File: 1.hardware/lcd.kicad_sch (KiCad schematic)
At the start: 36 parts, among them J6 FPC_LCD_40

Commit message: 중간 저장
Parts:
- PS1, PS2: footprint SOT65P210X110-5N -> SamacSys_Parts:SOT65P210X110-5N
- R12, R13, R14, R15, R16, R17, R18, R19, R20, R21, R22, R23, R24, R25, R26, R27, R28, R29, R30, R31, R32, R33: footprint (none) -> Resistor_SMD:R_0402_1005Metric
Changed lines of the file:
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@@
 			)
 		)
-		(property "Footprint" ""
+		(property "Footprint" "Resistor_SMD:R_0402_1005Metric"
 			(at 204.47 48.26 0)
 			(effects
@@
 			)
 		)
-		(property "Footprint" ""
+		(property "Footprint" "Resistor_SMD:R_0402_1005Metric"
 			(at 204.47 50.8 0)
 			(effects
@@
 			)
 		)
-		(property "Footprint" ""
+		(property "Footprint" "Resistor_SMD:R_0402_1005Metric"
 			(at 204.47 78.74 0)
 			(effects
@@
 			)
 		)
-		(property "Footprint" ""
+		(property "Footprint" "Resistor_SMD:R_0402_1005Metric"
 			(at 204.47 66.04 0)
 			(effects
@@
 			)
 		)
-		(property "Footprint" ""
+		(property "Footprint" "Resistor_SMD:R_0402_1005Metric"
 			(at 204.47 81.28 0)
 			(effects
@@
 			)
 		)
-		(property "Footprint" ""
+		(property "Footprint" "Resistor_SMD:R_0402_1005Metric"
 			(at 204.47 76.2 0)
 			(effects
@@
 			)
 		)
-		(property "Footprint" ""
+		(property "Footprint" "Resistor_SMD:R_0402_1005Metric"
 			(at 204.47 99.06 0)
 			(effects
@@
 			)
 		)
-		(property "Footprint" ""
+		(property "Footprint" "Resistor_SMD:R_0402_1005Metric"
 			(at 204.47 60.96 0)
 			(effects
@@
 			)
 		)
-		(property "Footprint" ""
+		(property "Footprint" "Resistor_SMD:R_0402_1005Metric"
 			(at 204.47 58.42 0)
 			(effects
@@
 			)
 		)
-		(property "Footprint" ""
+		(property "Footprint" "Resistor_SMD:R_0402_1005Metric"
 			(at 204.47 88.9 0)
 			(effects
@@
 			)
 		)
-		(property "Footprint" ""
+		(property "Footprint" "Resistor_SMD:R_0402_1005Metric"
 			(at 204.47 71.12 0)
 			(effects
@@
 			)
 		)
-		(property "Footprint" "SOT65P210X110-5N"
+		(property "Footprint" "SamacSys_Parts:SOT65P210X110-5N"
 			(at 101.6 69.85 0)
 			(effects
@@
 			)
 		)
-		(property "Footprint" ""
+		(property "Footprint" "Resistor_SMD:R_0402_1005Metric"
 			(at 204.47 55.88 0)
 			(effects
@@
 			)
 		)
-		(property "Footprint" ""
+		(property "Footprint" "Resistor_SMD:R_0402_1005Metric"
 			(at 204.47 86.36 0)
 			(effects
@@
 			)
 		)
-		(property "Footprint" ""
+		(property "Footprint" "Resistor_SMD:R_0402_1005Metric"
 			(at 204.47 101.6 0)
 			(effects
@@
 			)
 		)
-		(property "Footprint" "SOT65P210X110-5N"
+		(property "Footprint" "SamacSys_Parts:SOT65P210X110-5N"
 			(at 101.6 39.37 0)
 			(effects
@@
 			)
 		)
-		(property "Footprint" ""
+		(property "Footprint" "Resistor_SMD:R_0402_1005Metric"
 			(at 204.47 68.58 0)
 			(effects
@@
 			)
 		)
-		(property "Footprint" ""
+		(property "Footprint" "Resistor_SMD:R_0402_1005Metric"
 			(at 204.47 106.68 0)
 			(effects
@@
 			)
 		)
-		(property "Footprint" ""
+		(property "Footprint" "Resistor_SMD:R_0402_1005Metric"
 			(at 204.47 53.34 0)
 			(effects
@@
 			)
 		)
-		(property "Footprint" ""
+		(property "Footprint" "Resistor_SMD:R_0402_1005Metric"
 			(at 204.47 63.5 0)
 			(effects
@@
 			)
 		)
-		(property "Footprint" ""
+		(property "Footprint" "Resistor_SMD:R_0402_1005Metric"
 			(at 204.47 93.98 0)
 			(effects
@@
 			)
 		)
-		(property "Footprint" ""
+		(property "Footprint" "Resistor_SMD:R_0402_1005Metric"
 			(at 204.47 83.82 0)
 			(effects
@@
 			)
 		)
-		(property "Footprint" ""
+		(property "Footprint" "Resistor_SMD:R_0402_1005Metric"
 			(at 204.47 96.52 0)
 			(effects
@@
 			)
 		)
-		(property "Footprint" ""
+		(property "Footprint" "Resistor_SMD:R_0402_1005Metric"
 			(at 204.47 104.14 0)
 			(effects

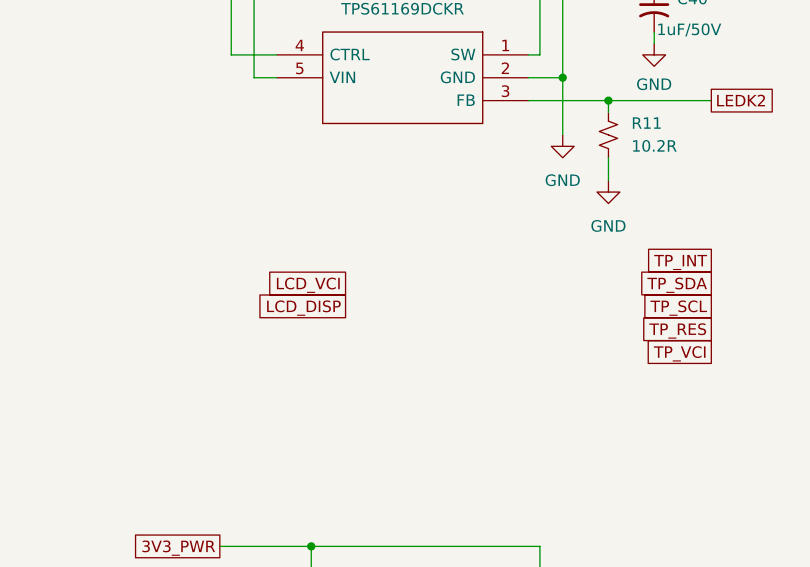
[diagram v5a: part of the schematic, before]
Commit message: 중간 수정
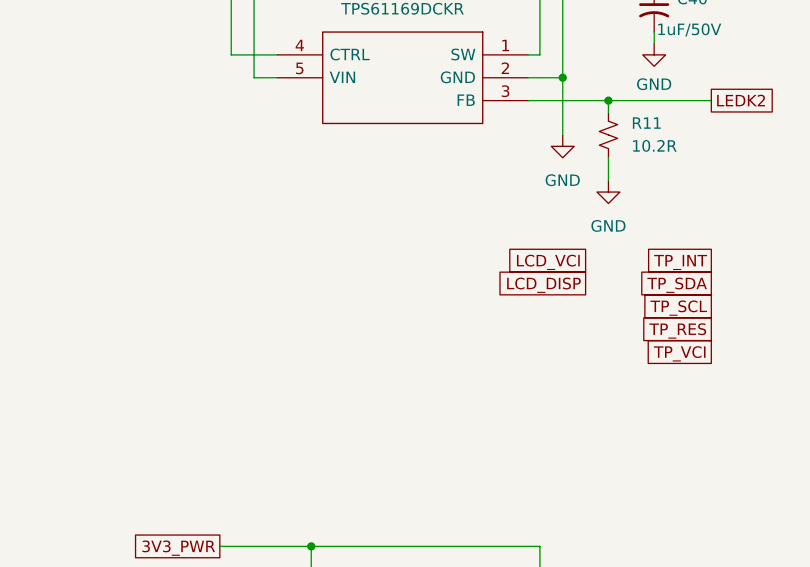
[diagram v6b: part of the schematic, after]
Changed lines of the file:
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@@
 	(global_label "LCD_VCI"
 		(shape passive)
-		(at 105.41 97.79 180)
-		(fields_autoplaced yes)
-		(effects
-			(font
-				(size 1.27 1.27)
-			)
-			(justify right)
-		)
-		(property "Intersheetrefs" "${INTERSHEET_REFS}"
-			(at 96.037 97.79 0)
+		(at 132.08 95.25 180)
+		(fields_autoplaced yes)
+		(effects
+			(font
+				(size 1.27 1.27)
+			)
+			(justify right)
+		)
+		(property "Intersheetrefs" "${INTERSHEET_REFS}"
+			(at 122.707 95.25 0)
 			(effects
 				(font
@@
 	(global_label "LCD_DISP"
 		(shape passive)
-		(at 105.41 100.33 180)
-		(fields_autoplaced yes)
-		(effects
-			(font
-				(size 1.27 1.27)
-			)
-			(justify right)
-		)
-		(property "Intersheetrefs" "${INTERSHEET_REFS}"
-			(at 94.6461 100.33 0)
-			(effects
-				(font
+		(at 132.08 97.79 180)
+		(fields_autoplaced yes)
+		(effects
+			(font
+				(size 1.27 1.27)
+			)
+			(justify right)
+		)
+		(property "Intersheetrefs" "${INTERSHEET_REFS}"
+			(at 121.3161 97.79 0)
+			(effects
+				(font
